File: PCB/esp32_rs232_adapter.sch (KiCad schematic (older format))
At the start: 25 parts, among them J1 Conn_01x04_Male, J2 DB9, SW1 Flash, SW2 Null_Modem_Selector, U1 ESP32-WROOM-32D, U2 MAX3232

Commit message: update
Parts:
- removed J1: Conn_01x04_Male, Connector_PinHeader_2.54mm:PinHeader_1x04_P2.54mm_Vertical, symbol Connector:Conn_01x04_Male
- U2: footprint Package_SO:SSOP-16_5.3x6.2mm_P0.65mm -> Package_SO:SOP-16_4.55x10.3mm_P1.27mm
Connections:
- wire segments 121 -> 126
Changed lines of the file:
@@
 EESchema Schematic File Version 4
 LIBS:esp32_rs232_adapter-cache
-EELAYER 26 0
+EELAYER 29 0
 EELAYER END
 $Descr A4 11693 8268
@@
 F 0 "U2" H 9000 4578 50  0000 C CNN
 F 1 "MAX3232" H 9000 4487 50  0000 C CNN
-F 2 "Package_SO:SSOP-16_5.3x6.2mm_P0.65mm" H 9050 2150 50  0001 L CNN
+F 2 "Package_SO:SOP-16_4.55x10.3mm_P1.27mm" H 9050 2150 50  0001 L CNN
 F 3 "https://datasheets.maximintegrated.com/en/ds/MAX3222-MAX3241.pdf" H 9000 3300 50  0001 C CNN
 F 4 "https://www.aliexpress.com/item/in-stock-can-pay-MAX3232CSE-MAX3232-MAX3232ESE-SOP-16/32821460559.html" H 9000 3200 50  0001 C CNN "Supplier"
@@
 F2 "3.3V" I R 3950 2500 50
 F3 "Vbatt_sig" I R 3950 2800 50
+F4 "power_status" I R 3950 3050 50
+F5 "charge_status" I R 3950 3150 50
 $EndSheet
 Wire Wire Line
@@
 Wire Wire Line
 	3950 2800 5400 2800
-$Comp
-L Connector:Conn_01x04_Male J1
-U 1 1 5C7F4A31
-P 2700 4350
-F 0 "J1" H 2806 4628 50  0000 C CNN
-F 1 "Conn_01x04_Male" H 2806 4537 50  0000 C CNN
-F 2 "Connector_PinHeader_2.54mm:PinHeader_1x04_P2.54mm_Vertical" H 2700 4350 50  0001 C CNN
-F 3 "~" H 2700 4350 50  0001 C CNN
-	1    2700 4350
-	1    0    0    -1
-$EndComp
-Wire Wire Line
-	2900 4250 3350 4250
-Wire Wire Line
-	2900 4350 3350 4350
-Wire Wire Line
-	2900 4550 3350 4550
-$Comp
-L power:GND #PWR01
-U 1 1 5C8018A8
-P 3350 4600
-F 0 "#PWR01" H 3350 4350 50  0001 C CNN
-F 1 "GND" H 3355 4427 50  0000 C CNN
-F 2 "" H 3350 4600 50  0001 C CNN
-F 3 "" H 3350 4600 50  0001 C CNN
-	1    3350 4600
-	1    0    0    -1
-$EndComp
-Wire Wire Line
-	3350 4600 3350 4550
-$Comp
-L power:+3.3V #PWR02
-U 1 1 5C804F12
-P 3550 4450
-F 0 "#PWR02" H 3550 4300 50  0001 C CNN
-F 1 "+3.3V" H 3565 4623 50  0000 C CNN
-F 2 "" H 3550 4450 50  0001 C CNN
-F 3 "" H 3550 4450 50  0001 C CNN
-	1    3550 4450
-	1    0    0    -1
-$EndComp
-Wire Wire Line
-	2900 4450 3550 4450
-Text Label 3350 4350 2    50   ~ 0
-TXD
-Text Label 3350 4250 2    50   ~ 0
-RXD
 $Comp
 L Device:LED_Small D3
@@
 	1    0    0    -1
 $EndComp
+Wire Wire Line
+	3950 3050 4800 3050
+Wire Wire Line
+	4800 3050 4800 5400
+Wire Wire Line
+	4800 5400 6700 5400
+Wire Wire Line
+	6700 5400 6700 4900
+Wire Wire Line
+	6700 4900 6600 4900
+Wire Wire Line
+	3950 3150 4700 3150
+Wire Wire Line
+	4700 3150 4700 5500
+Wire Wire Line
+	4700 5500 6750 5500
+Wire Wire Line
+	6750 5500 6750 4800
+Wire Wire Line
+	6750 4800 6600 4800
 $EndSCHEMATC

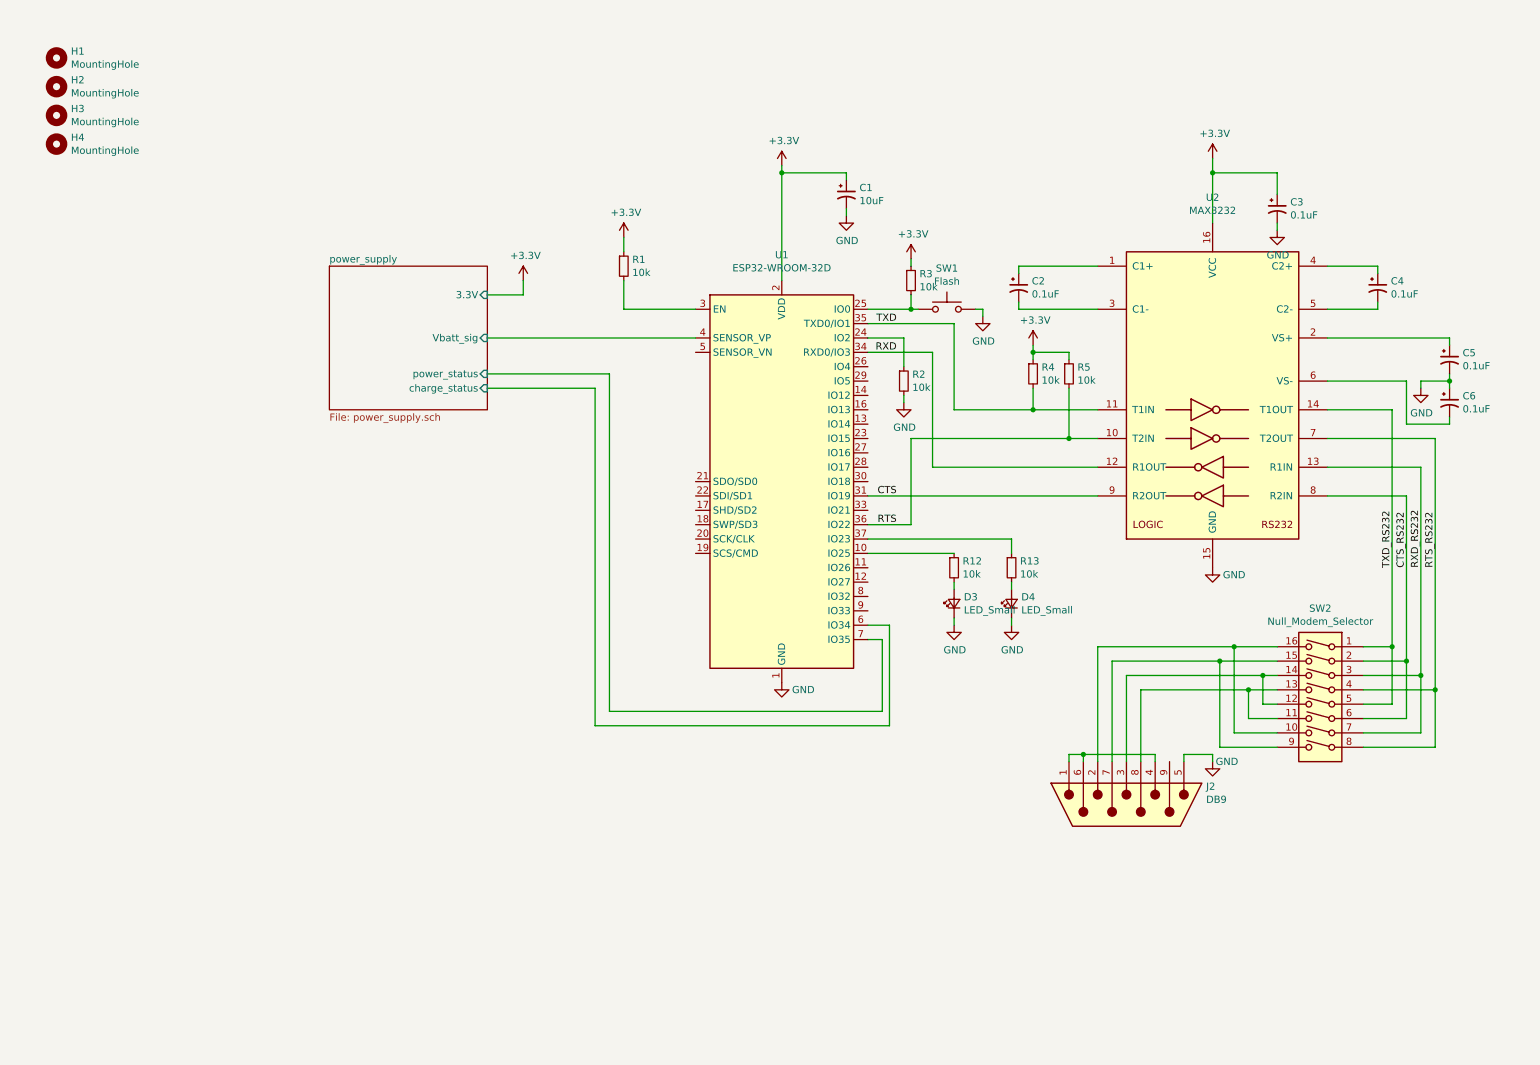
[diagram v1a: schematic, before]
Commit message: work in progress with stuff for cb testing
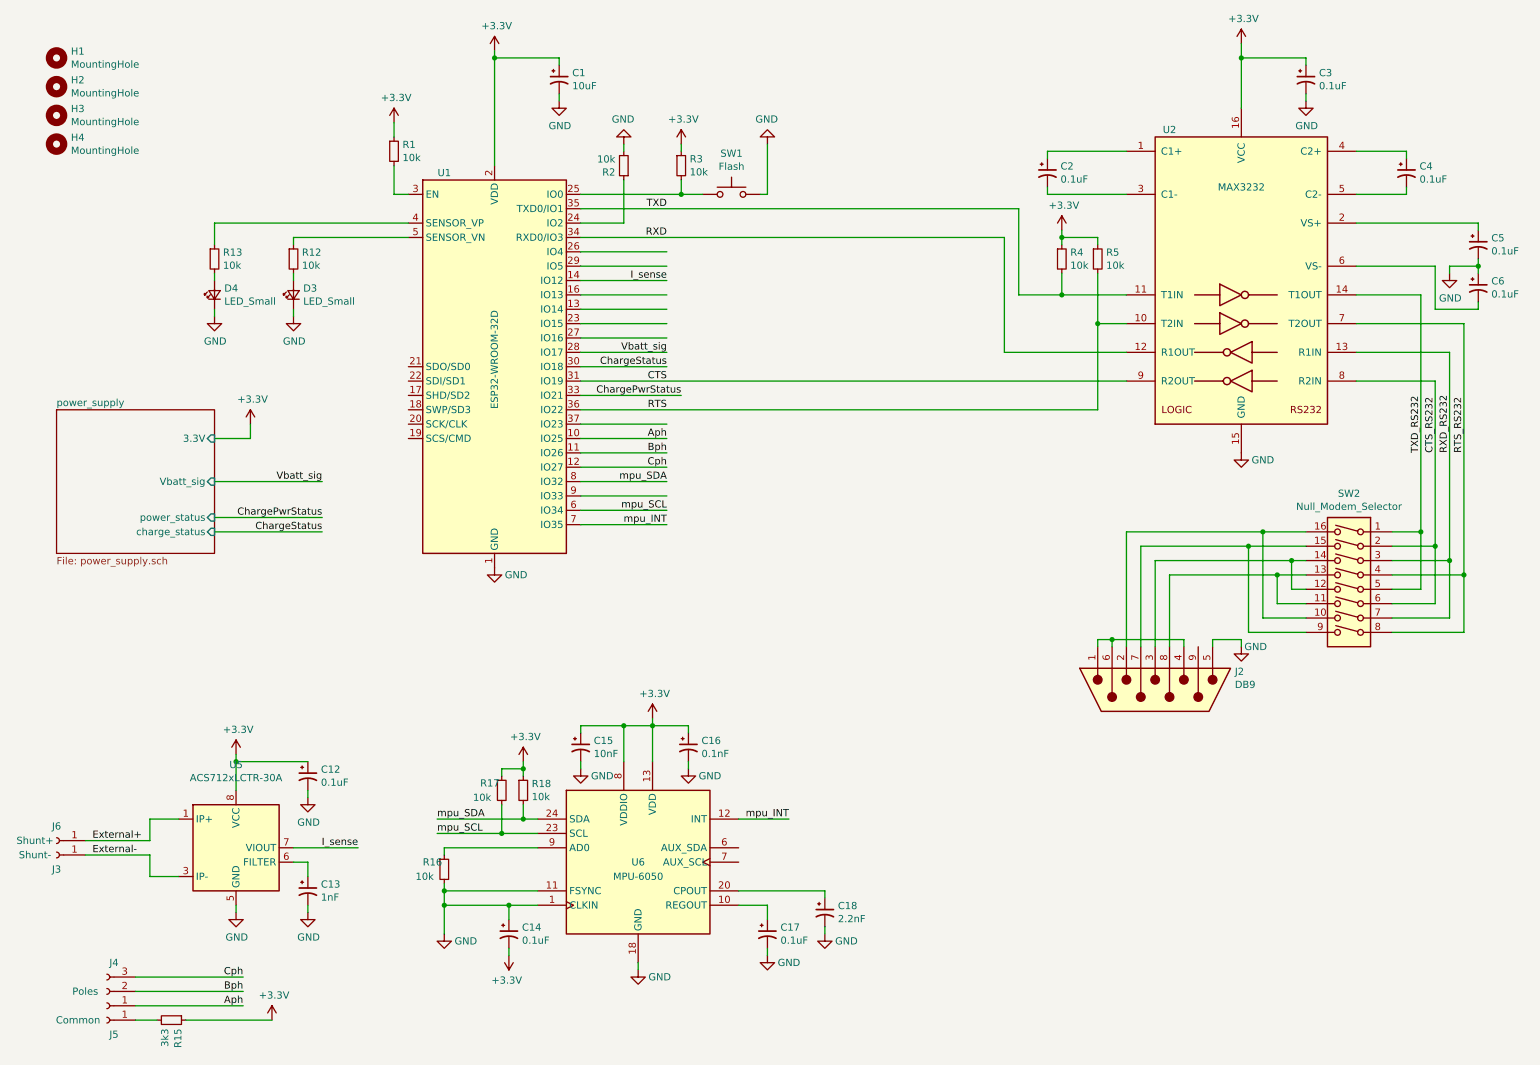
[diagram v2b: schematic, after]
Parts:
- added C12, C14, C17: 0.1uF, Capacitor_SMD:C_0805_2012Metric, symbol Device:CP1_Small
- added C13: 1nF, Capacitor_SMD:C_0805_2012Metric, symbol Device:CP1_Small
- added C15: 10nF, Capacitor_SMD:C_0805_2012Metric, symbol Device:CP1_Small
- added C16: 0.1nF, Capacitor_SMD:C_0805_2012Metric, symbol Device:CP1_Small
- added C18: 2.2nF, Capacitor_SMD:C_0805_2012Metric, symbol Device:CP1_Small
- added J3: Shunt-, Connector:Banana_Jack_1Pin, symbol Connector:Conn_01x01_Female
- added J4: Poles, Connector:Banana_Jack_3Pin, symbol Connector:Conn_01x03_Female
- added J5: Common, Connector:Banana_Jack_1Pin, symbol Connector:Conn_01x01_Female
- added J6: Shunt+, Connector:Banana_Jack_1Pin, symbol Connector:Conn_01x01_Female
- added R15: 3k3, Resistor_SMD:R_0805_2012Metric, symbol Device:R_Small
- added R16, R17, R18: 10k, Resistor_SMD:R_0805_2012Metric, symbol Device:R_Small
- added U5: ACS712xLCTR-30A, Package_SO:SOIC-8_3.9x4.9mm_P1.27mm, symbol Sensor_Current:ACS712xLCTR-30A
- added U6: MPU-6050, Sensor_Motion:InvenSense_QFN-24_4x4mm_P0.5mm, symbol Sensor_Motion:MPU-6050
- U1: footprint RF_Module:ESP32-WROOM-32 -> power_supplies:ESP32-WROOM-32-Heat
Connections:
- net labels added: Aph, Bph, ChargePwrStatus, ChargeStatus, Cph, External+, External-, I_sense, Vbatt_sig, mpu_INT, mpu_SCL, mpu_SDA
- wire segments 126 -> 194
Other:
- moved on the sheet: C1, C2, C3, C4, C5, C6, D3, D4, J2, R1, R12, R13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
